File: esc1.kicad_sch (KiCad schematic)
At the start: 68 parts, among them J3 Pad Terminals, J4 Signal, Q1 NMOS, Q2 NMOS, Q3 NMOS, Q4 NMOS, Q5 NMOS, Q6 NMOS, U10 INA180A3, U11 IRS21867S, U12 INA180A3, U13 STM32F303CBTx, U7 IRS21867S, U8 INA180A3, U9 IRS21867S

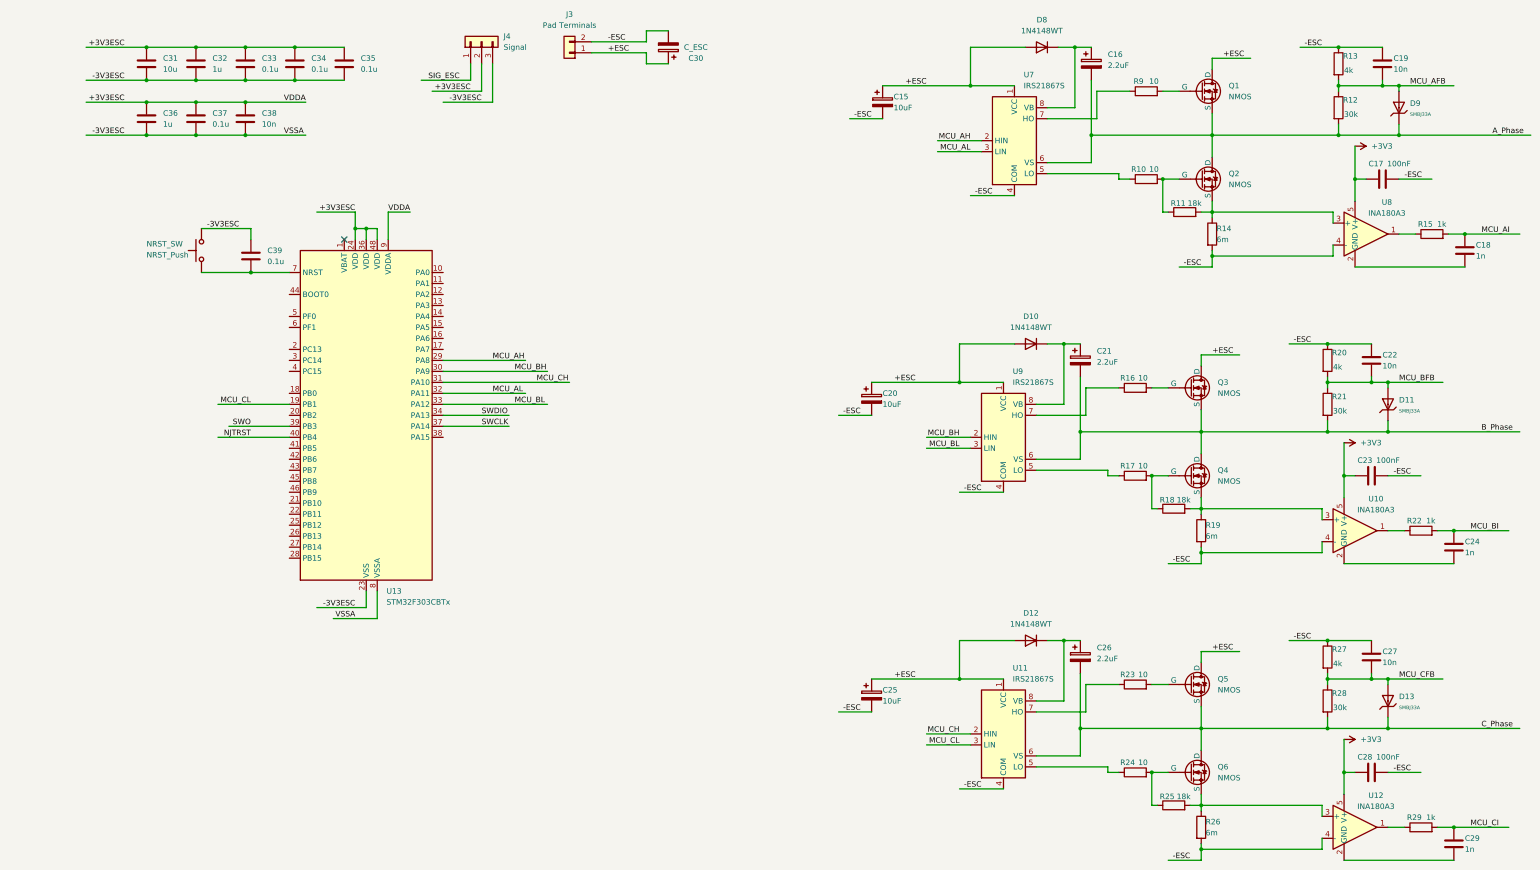
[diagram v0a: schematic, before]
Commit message: ESC Schematic Update
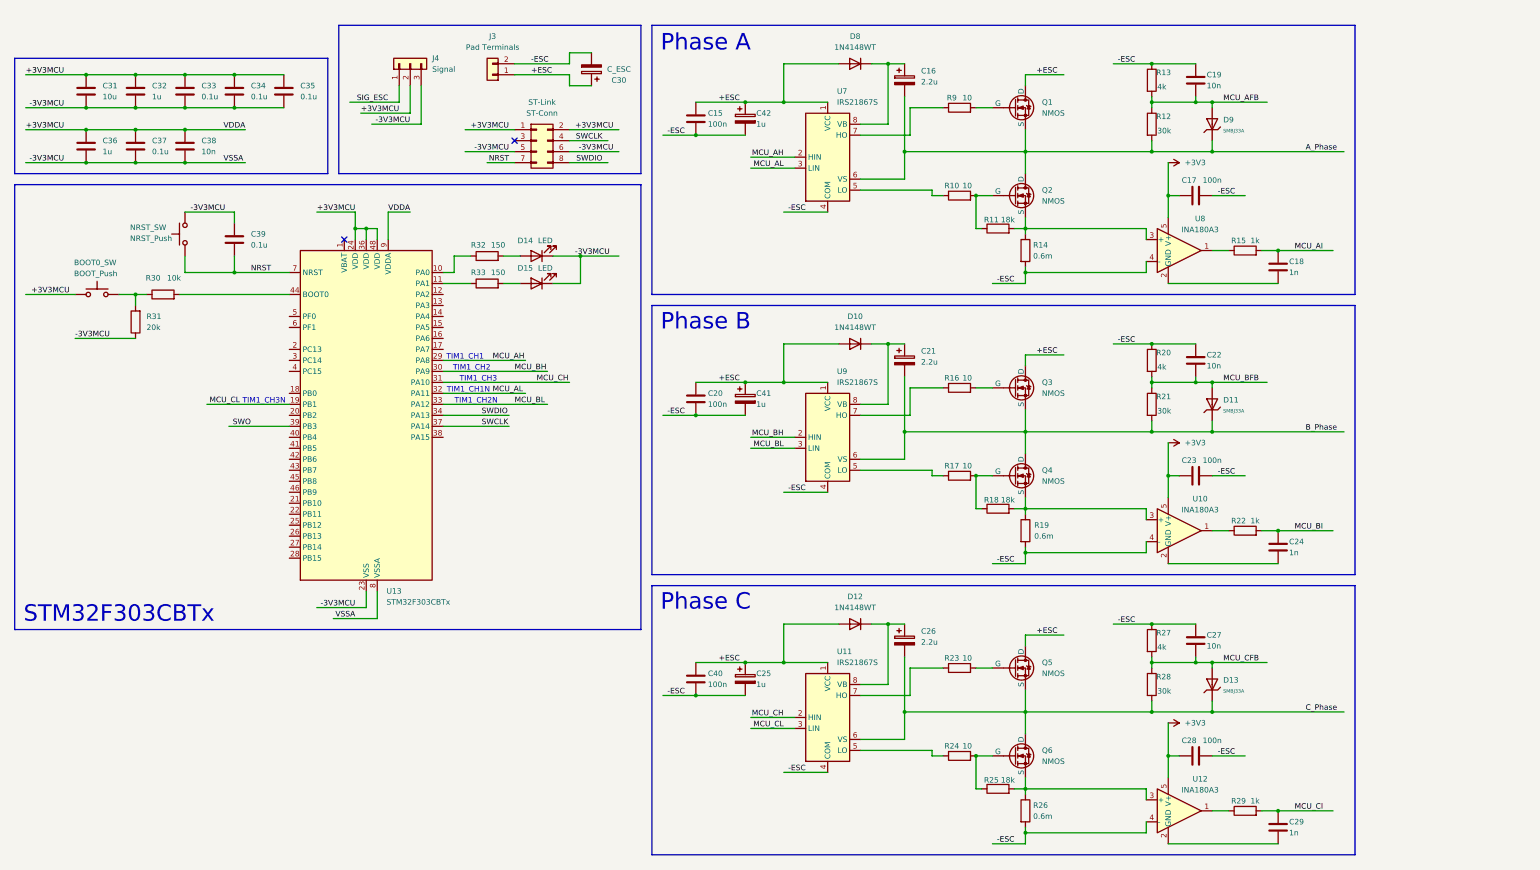
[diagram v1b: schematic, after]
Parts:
- removed C15, C20: 10uF, symbol Device:C_Polarized
- added BOOT0_SW: BOOT_Push, symbol Switch:SW_Push
- added C15, C20, C40: 100n, symbol Device:C
- added C41, C42: 1u, symbol Device:C_Polarized
- added D14, D15: LED, symbol Device:LED
- added R30: 10k, symbol Device:R
- added R31: 20k, symbol Device:R
- added R32, R33: 150, symbol Device:R
- added ST-Link: ST-Conn, symbol Connector_Generic:Conn_02x04_Odd_Even
- C16, C21, C26: value 2.2uF -> 2.2u
- C17, C23, C28: value 100nF -> 100n
- C25: value 10uF -> 1u
- R14, R19, R26: value 6m -> 0.6m
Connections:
- net +ESC: now also C15.1, C20.1, C40.1, C41.1, C42.1
- net -ESC: now also C15.2, C20.2, C40.2, C41.2, C42.2
- net SWCLK: now also ST-Link.4 (Pin_4)
- net SWDIO: now also ST-Link.8 (Pin_8)
- net NRST: now reaches C39.2, NRST_SW.1, U13.7 (NRST)
- net NRST: now also ST-Link.7 (Pin_7)
- net at U13.10 (PA0): now also R32.1
- net at U13.11 (PA1): now also R33.1
- net at U13.44 (BOOT0): now also R30.2
- net +3V3ESC renamed +3V3MCU
- net +3V3MCU: now also BOOT0_SW.1, ST-Link.1 (Pin_1), ST-Link.2 (Pin_2)
- net -3V3ESC renamed -3V3MCU
- net -3V3MCU: now also D14.1 (K), D15.1 (K), R31.1, ST-Link.5 (Pin_5), ST-Link.6 (Pin_6)
- net NJTRST: no longer names the net of U13.40 (PB4)
- new net: BOOT0_SW.2, R30.1, R31.2
- new net: D14.2 (A), R32.2
- new net: D15.2 (A), R33.2
- no-connect marks 1 -> 2
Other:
- note added: "Phase A"
- note added: "Phase B"
- note added: "Phase C"
- note added: "STM32F303CBTx"
- note added: "TIM1_CH1"
- note added: "TIM1_CH1N"
- note added: "TIM1_CH2"
- note added: "TIM1_CH2N"
- note added: "TIM1_CH3"
- note added: "TIM1_CH3N"
- moved on the sheet: C16, C17, C18, C19, C21, C22, C23, C24, C25, C26, C27, C28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
